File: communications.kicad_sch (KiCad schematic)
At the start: 13 parts, among them CN1 PJ-3059-B, U41 DSLVDS1048PWR, U42 DSLVDS1047PWR

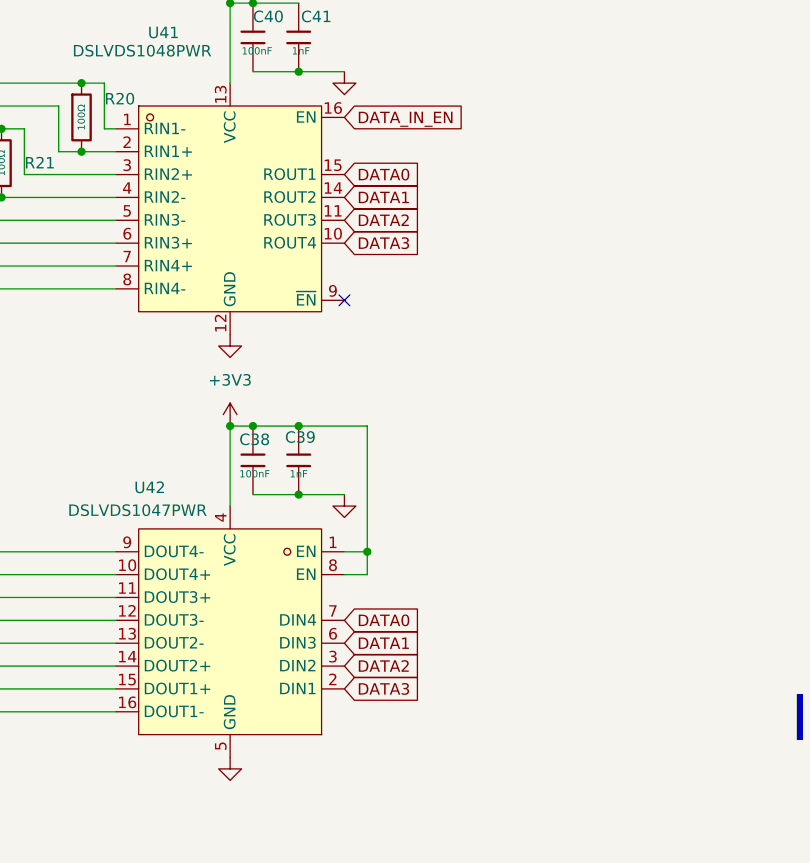
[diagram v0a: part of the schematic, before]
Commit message: Checkpoint
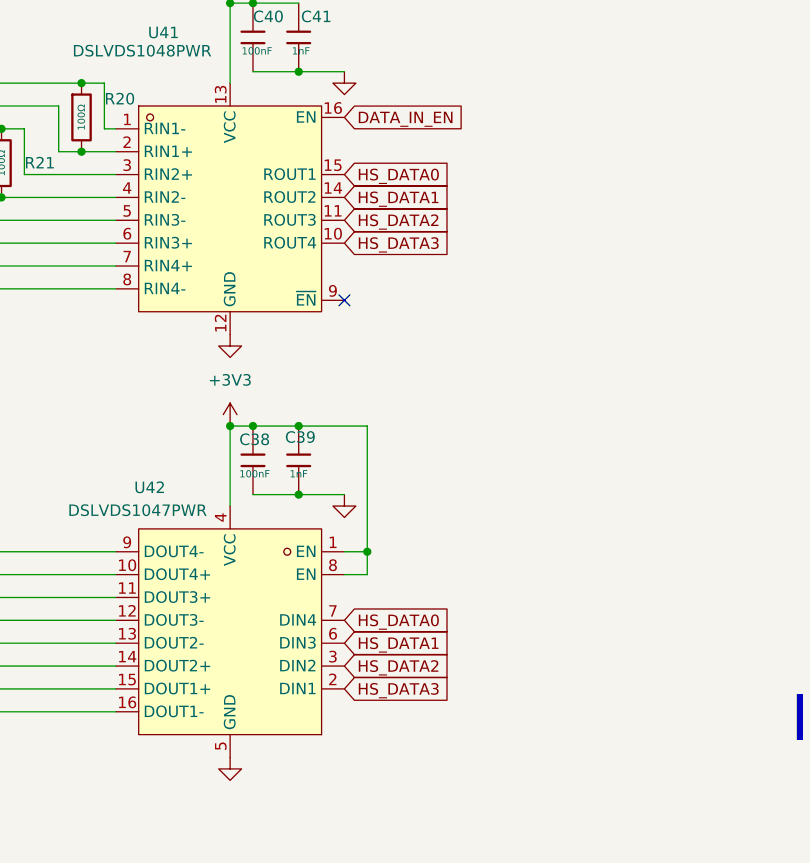
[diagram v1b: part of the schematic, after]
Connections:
- net DATA0 renamed HS_DATA0
- net DATA1 renamed HS_DATA1
- net DATA2 renamed HS_DATA2
- net DATA3 renamed HS_DATA3
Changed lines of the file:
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@@
 		)
 	)
-	(global_label "DATA1"
+	(global_label "HS_DATA1"
 		(shape input)
 		(at 167.64 116.84 0)
@@
 		)
 		(property "Intersheetrefs" "${INTERSHEET_REFS}"
-			(at 176.2495 116.84 0)
-			(effects
-				(font
-					(size 1.27 1.27)
-				)
-				(justify left)
-				(hide yes)
-			)
-		)
-	)
-	(global_label "DATA3"
+			(at 179.7571 116.84 0)
+			(effects
+				(font
+					(size 1.27 1.27)
+				)
+				(justify left)
+				(hide yes)
+			)
+		)
+	)
+	(global_label "HS_DATA3"
 		(shape input)
 		(at 167.64 121.92 0)
@@
 		)
 		(property "Intersheetrefs" "${INTERSHEET_REFS}"
-			(at 176.2495 121.92 0)
-			(effects
-				(font
-					(size 1.27 1.27)
-				)
-				(justify left)
-				(hide yes)
-			)
-		)
-	)
-	(global_label "DATA0"
+			(at 179.7571 121.92 0)
+			(effects
+				(font
+					(size 1.27 1.27)
+				)
+				(justify left)
+				(hide yes)
+			)
+		)
+	)
+	(global_label "HS_DATA0"
 		(shape input)
 		(at 167.64 114.3 0)
@@
 		)
 		(property "Intersheetrefs" "${INTERSHEET_REFS}"
-			(at 176.2495 114.3 0)
-			(effects
-				(font
-					(size 1.27 1.27)
-				)
-				(justify left)
-				(hide yes)
-			)
-		)
-	)
-	(global_label "DATA1"
+			(at 179.7571 114.3 0)
+			(effects
+				(font
+					(size 1.27 1.27)
+				)
+				(justify left)
+				(hide yes)
+			)
+		)
+	)
+	(global_label "HS_DATA1"
 		(shape input)
 		(at 167.64 67.31 0)
@@
 		)
 		(property "Intersheetrefs" "${INTERSHEET_REFS}"
-			(at 176.2495 67.31 0)
+			(at 179.7571 67.31 0)
 			(effects
 				(font
@@
 		)
 	)
-	(global_label "DATA2"
+	(global_label "HS_DATA2"
 		(shape input)
 		(at 167.64 69.85 0)
@@
 		)
 		(property "Intersheetrefs" "${INTERSHEET_REFS}"
-			(at 176.2495 69.85 0)
+			(at 179.7571 69.85 0)
 			(effects
 				(font
@@
 		)
 	)
-	(global_label "DATA3"
+	(global_label "HS_DATA3"
 		(shape input)
 		(at 167.64 72.39 0)
@@
 		)
 		(property "Intersheetrefs" "${INTERSHEET_REFS}"
-			(at 176.2495 72.39 0)
-			(effects
-				(font
-					(size 1.27 1.27)
-				)
-				(justify left)
-				(hide yes)
-			)
-		)
-	)
-	(global_label "DATA2"
+			(at 179.7571 72.39 0)
+			(effects
+				(font
+					(size 1.27 1.27)
+				)
+				(justify left)
+				(hide yes)
+			)
+		)
+	)
+	(global_label "HS_DATA2"
 		(shape input)
 		(at 167.64 119.38 0)
@@
 		)
 		(property "Intersheetrefs" "${INTERSHEET_REFS}"
-			(at 176.2495 119.38 0)
-			(effects
-				(font
-					(size 1.27 1.27)
-				)
-				(justify left)
-				(hide yes)
-			)
-		)
-	)
-	(global_label "DATA0"
+			(at 179.7571 119.38 0)
+			(effects
+				(font
+					(size 1.27 1.27)
+				)
+				(justify left)
+				(hide yes)
+			)
+		)
+	)
+	(global_label "HS_DATA0"
 		(shape input)
 		(at 167.64 64.77 0)
@@
 		)
 		(property "Intersheetrefs" "${INTERSHEET_REFS}"
-			(at 176.2495 64.77 0)
-			(effects
-				(font
+			(at 179.7571 64.77 0)
+			(effects
+				(font

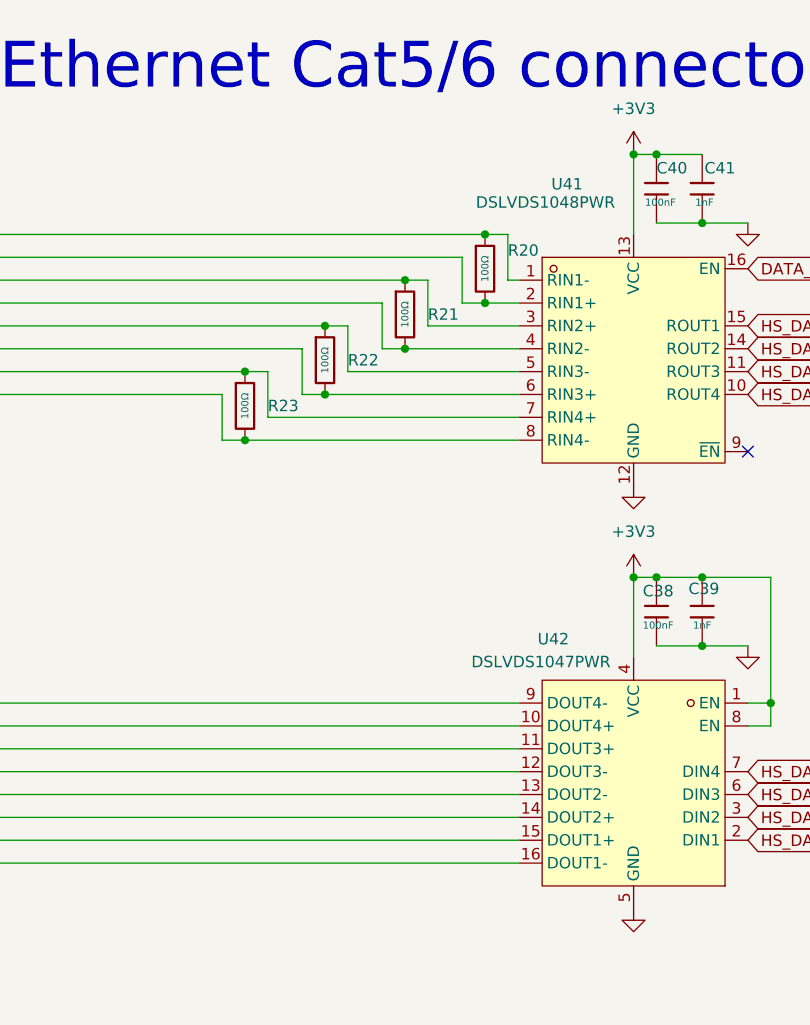
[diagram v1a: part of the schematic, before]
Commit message: Checkpoint
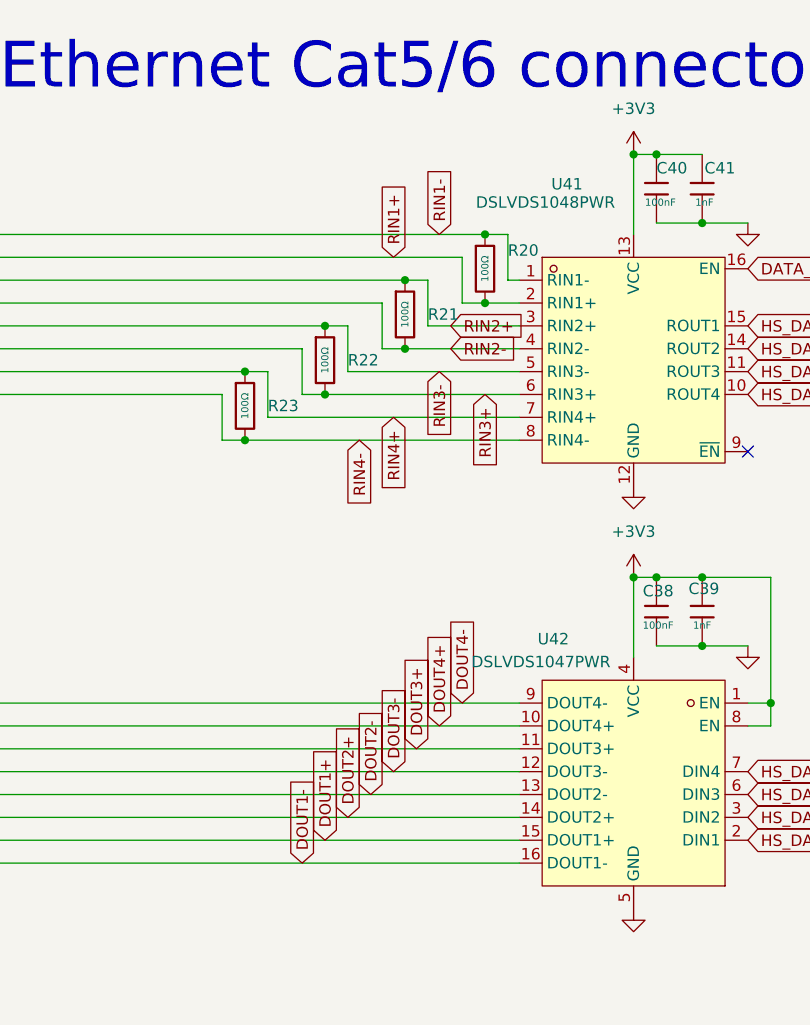
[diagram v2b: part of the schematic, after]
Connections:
- net DOUT1-: now reaches RJ2.1, U42.16 (DOUT1-)
- net DOUT1+: now reaches RJ2.2, U42.15 (DOUT1+)
- net DOUT2+: now reaches RJ2.3, U42.14 (DOUT2+)
- net DOUT2-: now reaches RJ2.4, U42.13 (DOUT2-)
- net DOUT3-: now reaches RJ2.5, U42.12 (DOUT3-)
- net DOUT3+: now reaches RJ2.6, U42.11 (DOUT3+)
- net DOUT4+: now reaches RJ2.7, U42.10 (DOUT4+)
- net DOUT4-: now reaches RJ2.8, U42.9 (DOUT4-)
- net RIN1-: now reaches R20.1, RJ1.8, U41.1 (RIN1-)
- net RIN1+: now reaches R20.2, RJ1.7, U41.2 (RIN1+)
- net RIN2+: now reaches R21.1, RJ1.6, U41.3 (RIN2+)
- net RIN2-: now reaches R21.2, RJ1.5, U41.4 (RIN2-)
- net RIN4+: now reaches R23.1, RJ1.2, U41.7 (RIN4+)
- net RIN4-: now reaches R23.2, RJ1.1, U41.8 (RIN4-)
- net RIN3-: now reaches R22.1, RJ1.4, U41.5 (RIN3-)
- net RIN3+: now reaches R22.2, RJ1.3, U41.6 (RIN3+)
